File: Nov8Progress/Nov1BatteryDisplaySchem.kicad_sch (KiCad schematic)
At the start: 25 parts, among them J1 FH34SRJ-24S-0.5SH_99_, J2 Screw_Terminal_2x2.54, Q2 ZXM61N03F, SW1 Button

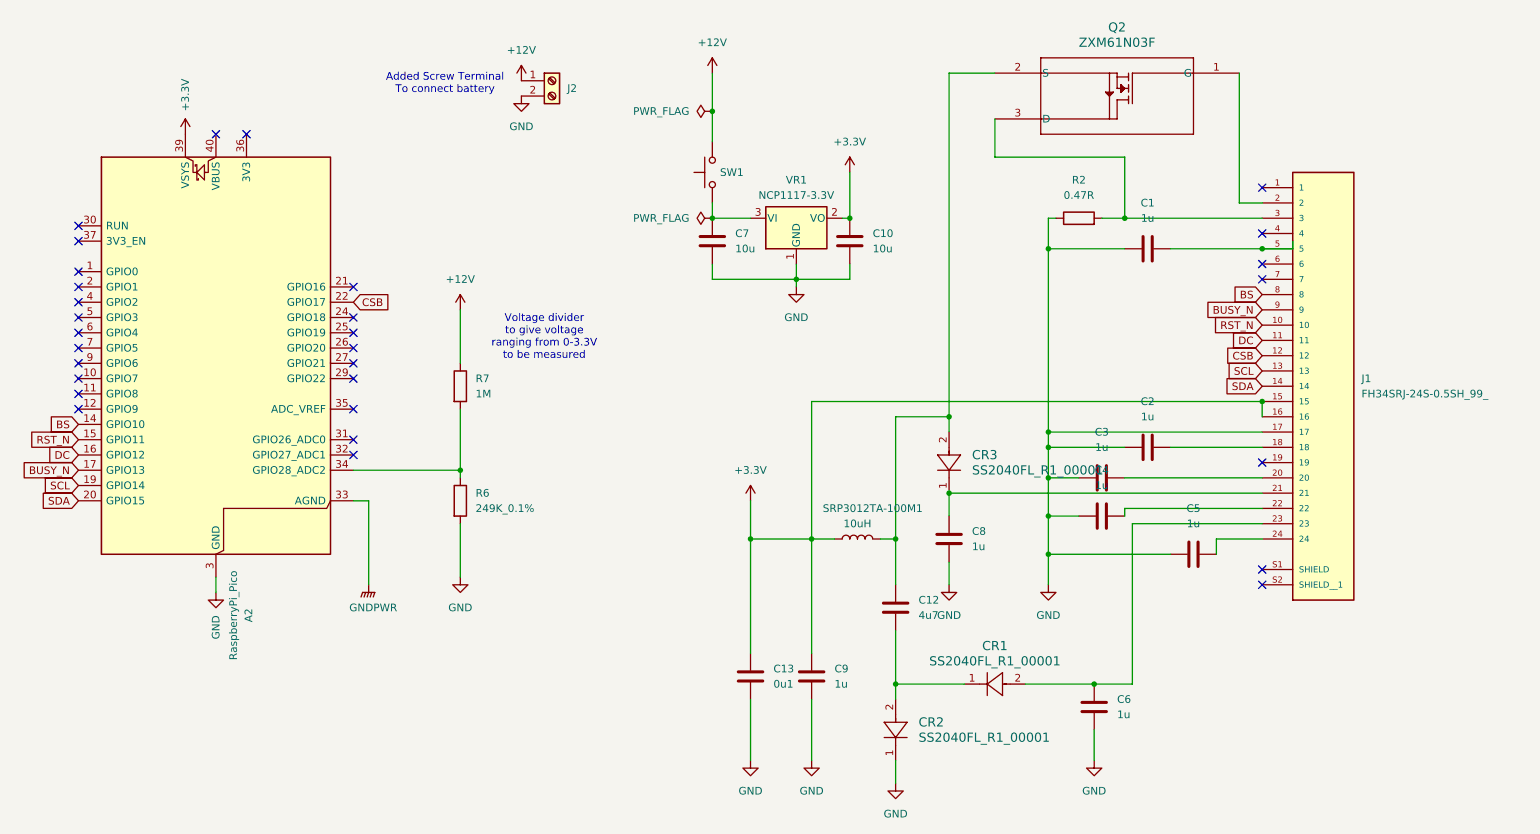
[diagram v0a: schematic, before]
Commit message: Jan10 Update
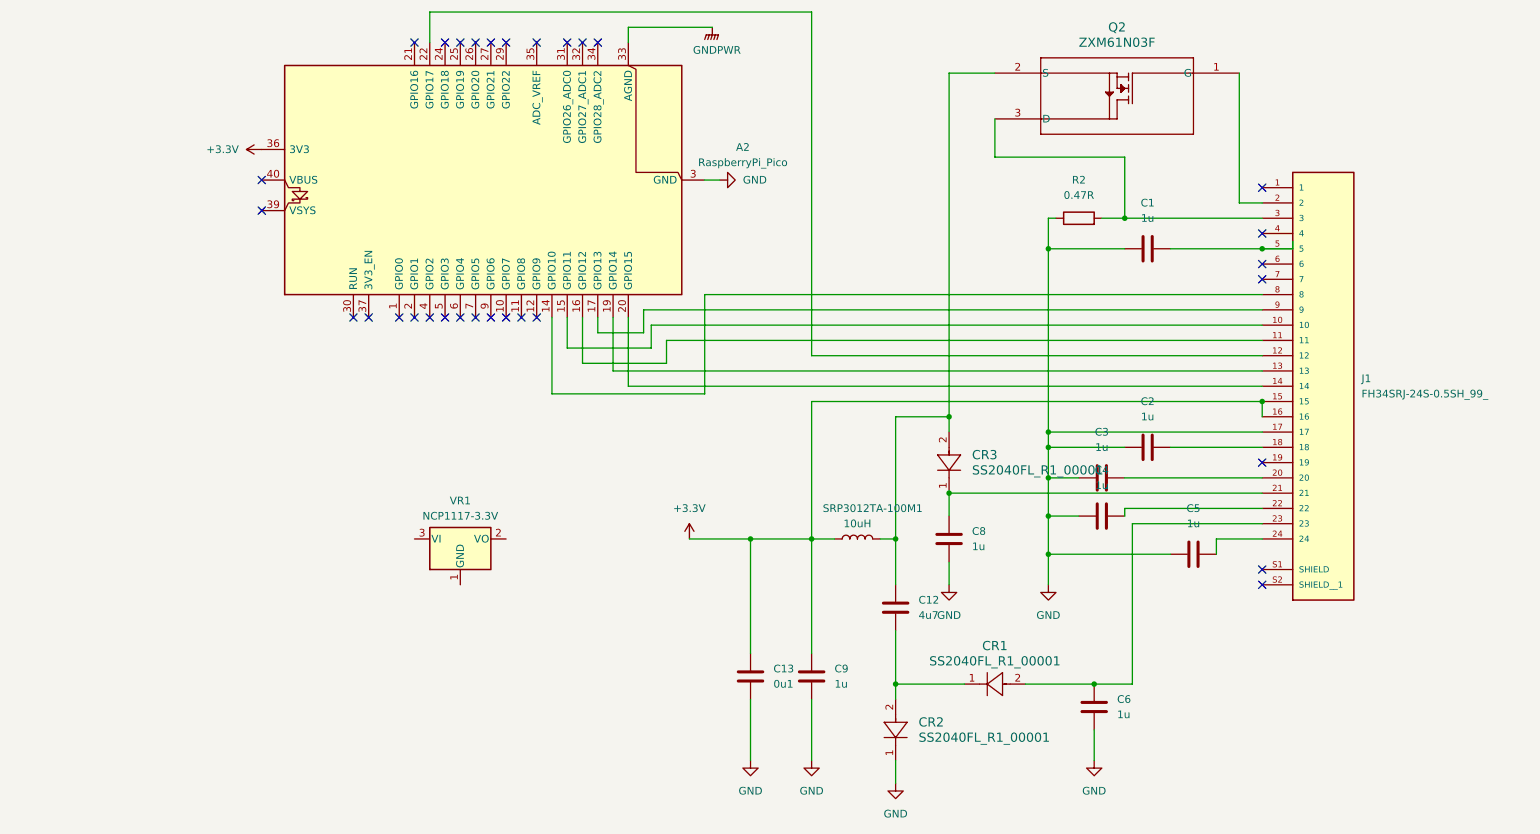
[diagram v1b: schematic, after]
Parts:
- removed C10, C7: 10u, rsx_capacitors:C_0805_2012Metric, symbol rsx_Capacitors:10u
- removed J2: Screw_Terminal_2x2.54, rsx_headers_screw:Wurth_691210910002, symbol rsx_header_screw:Screw_Terminal_2x2.54
- removed R6: 249K_0.1%, rsx_resistors:R_0603_1608Metric, symbol rsx_Resistors:249K_0.1%
- removed R7: 1M, rsx_resistors:R_0603_1608Metric, symbol rsx_Resistors:1M
- removed SW1: Button, rsx_HID:FSMSMTR, symbol rsx_HID:Button
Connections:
- net +3.3V: now also A2.36 (3V3); no longer A2.39 (VSYS), VR1.2 (VO)
- net GND: no longer VR1.1 (GND)
- net BS: no longer names the net of A2.14 (GPIO10), J1.8
- net BUSY_N: no longer names the net of A2.17 (GPIO13), J1.9
- net CSB: no longer names the net of A2.22 (GPIO17), J1.12
- net DC: no longer names the net of A2.16 (GPIO12), J1.11
- net RST_N: no longer names the net of A2.15 (GPIO11), J1.10
- net SCL: no longer names the net of A2.19 (GPIO14), J1.13
- net SDA: no longer names the net of A2.20 (GPIO15), J1.14
- no-connect marks 30 -> 31
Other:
- note removed: "Added Screw Terminal To connect battery"
- note removed: "Voltage divider to give voltage ranging from 0-3.3V to be measured"
- moved on the sheet: A2, VR1
